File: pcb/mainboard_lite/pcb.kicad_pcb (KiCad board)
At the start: 4 copper layers, 50 x 47 mm, 196 parts, among them J201 Conn_02x05_Odd_Even, J401 FH12-40S-0.5SH, J402 HDMI_A, J403 USB_C_Receptacle_USB2.0, J404 Power Switch, Q401 BSS138, Q402 BSS138, Q403 BSS138, Q404 BSS84, Q406 S8050W, U200 XC6SLX16-FTG256, U401 SY8120, U402 MT3608, U404 SY8120, U405 SY8120, U406 W25Q16JVP, U407 MT9700, U408 MT3608, U409 LGS5148, U410 LGS5148, U411 LM321, U502 MT41K64M16TW, Y201 33MHz

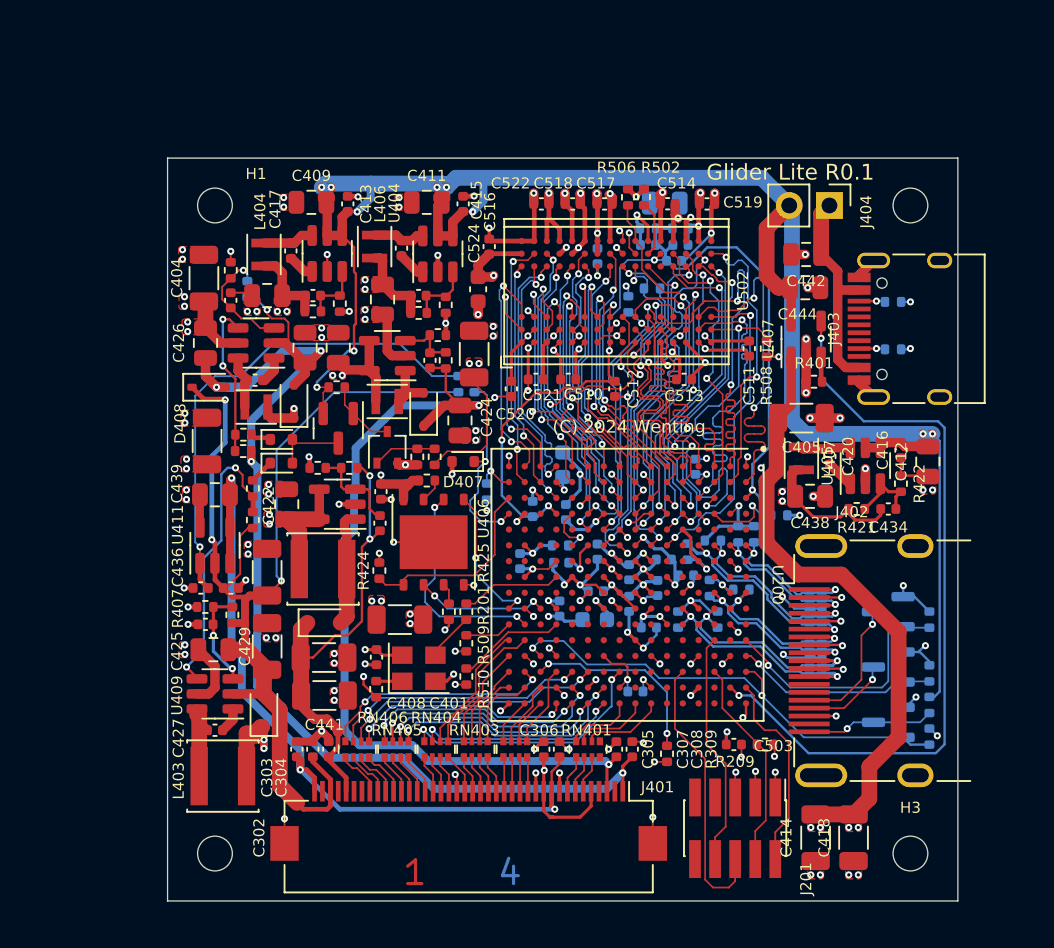
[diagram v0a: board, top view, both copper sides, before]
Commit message: Lite version r0p1
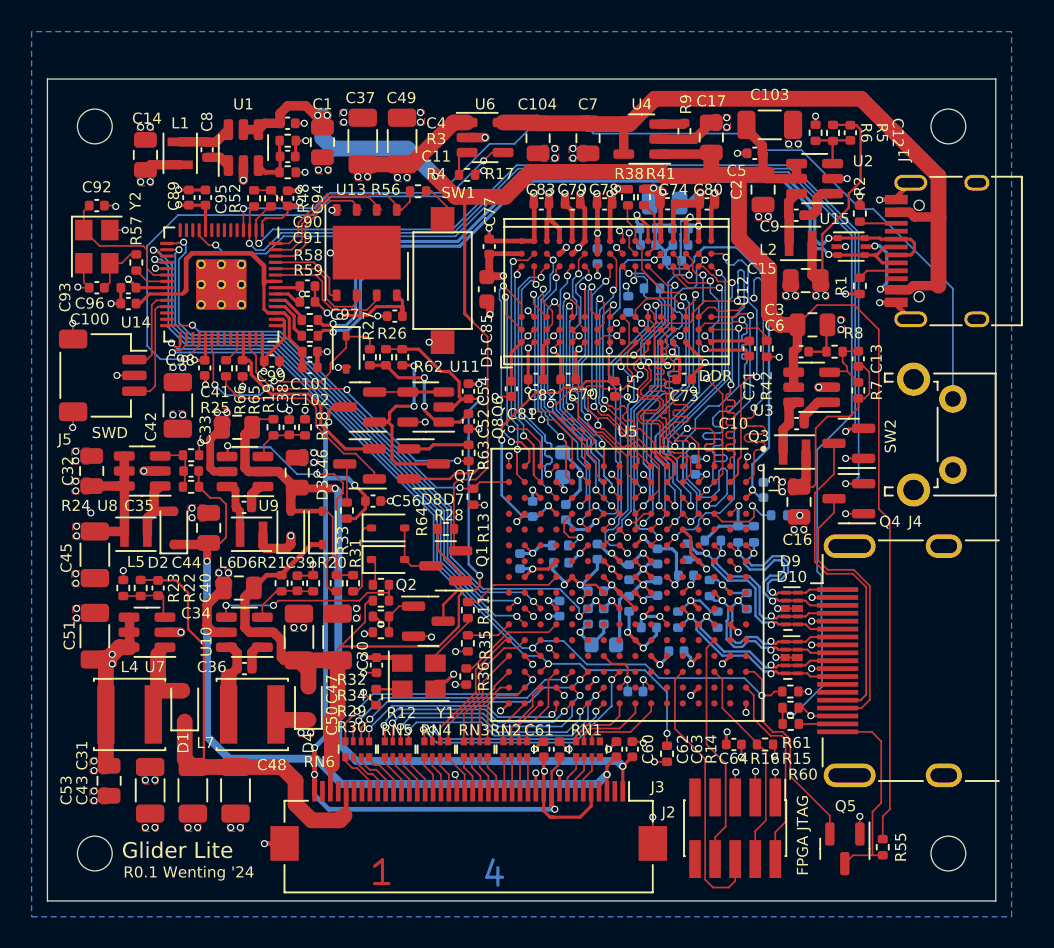
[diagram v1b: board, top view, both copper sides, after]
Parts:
- removed C302, C303, C304, C443: 220nF, Capacitor_SMD:C_0402_1005Metric
- removed C414: 47uF/10V, Capacitor_SMD:C_1206_3216Metric
- removed C442: 10uF/10V, Capacitor_SMD:C_0805_2012Metric
- removed J403: USB_C_Receptacle_USB2.0, Connector_USB:USB_C_Receptacle_HRO_TYPE-C-31-M-12
- removed J404: Power Switch, Connector_PinHeader_2.54mm:PinHeader_1x02_P2.54mm_Vertical
- removed Q401, Q402, Q403: BSS138, Package_TO_SOT_SMD:SOT-23
- removed Q404: BSS84, Package_TO_SOT_SMD:SOT-23
- removed R417, R418: 5.1K/1%, Resistor_SMD:R_0402_1005Metric
- removed R424: 10K/1%, Resistor_SMD:R_0402_1005Metric
- removed R425, R426: 4.7K, Resistor_SMD:R_0402_1005Metric
- removed R428: 1K/1%, Resistor_SMD:R_0402_1005Metric
- removed U402, U408: MT3608, Package_TO_SOT_SMD:TSOT-23-5
- removed U406: W25Q16JVP, Package_SON:WSON-8-1EP_6x5mm_P1.27mm_EP3.4x4.3mm
- added C100: 100nF, Capacitor_SMD:C_0402_1005Metric, F.Cu at (100.1, 62.2)
- added C101: 100nF, Capacitor_SMD:C_0402_1005Metric, F.Cu at (111.6, 65.2)
- added C102: 1uF, Capacitor_SMD:C_0402_1005Metric, F.Cu at (111.6, 66.2)
- added C103: 47uF/10V, Capacitor_SMD:C_1206_3216Metric, F.Cu at (140.7, 50.9)
- added C104: 10uF/10V, Capacitor_SMD:C_0805_2012Metric, F.Cu at (126.0, 51.8)
- added C57: 220nF, Capacitor_SMD:C_0402_1005Metric, B.Cu at (134.8, 84.2)
- added C58: 220nF, Capacitor_SMD:C_0402_1005Metric, B.Cu at (130.2, 82.0)
- added C59: 220nF, Capacitor_SMD:C_0402_1005Metric, B.Cu at (129.2, 82.0)
- added C7: 10uF/10V, Capacitor_SMD:C_0805_2012Metric, F.Cu at (129.2, 51.8)
- added C89: 1uF, Capacitor_SMD:C_0402_1005Metric, F.Cu at (104.0, 55.5)
- added C90: 100nF, Capacitor_SMD:C_0402_1005Metric, F.Cu at (111.5, 61.1)
- added C91: 100nF, Capacitor_SMD:C_0402_1005Metric, F.Cu at (111.5, 62.1)
- added C92: 18pF, Capacitor_SMD:C_0402_1005Metric, F.Cu at (98.1, 56.0)
- added C93: 18pF, Capacitor_SMD:C_0402_1005Metric, F.Cu at (98.1, 61.2)
- added C94: 100nF, Capacitor_SMD:C_0402_1005Metric, F.Cu at (110.2, 55.5)
- added C95: 100nF, Capacitor_SMD:C_0402_1005Metric, F.Cu at (105.0, 55.5)
- added C96: 100nF, Capacitor_SMD:C_0402_1005Metric, F.Cu at (100.1, 61.2)
- added C97: 100nF, Capacitor_SMD:C_0402_1005Metric, F.Cu at (117.0, 63.0)
- added C98: 100nF, Capacitor_SMD:C_0402_1005Metric, F.Cu at (105.0, 66.3)
- added C99: 100nF, Capacitor_SMD:C_0402_1005Metric, F.Cu at (109.2, 65.8)
- added J1: USB_C_Receptacle_USB2.0, Connector_USB:USB_C_Receptacle_HRO_TYPE-C-31-M-12, F.Cu at (152.8, 58.9)
- added J5: SM03B-SRSS-TB, Connector_JST:JST_SH_SM03B-SRSS-TB_1x03-1MP_P1.00mm_Horizontal, F.Cu at (98.5, 66.8)
- added Q1: AO3401A, Package_TO_SOT_SMD:SOT-23, F.Cu at (120.2, 78.8)
- added Q3: AO3400A, Package_TO_SOT_SMD:SOT-23, F.Cu at (145.7, 71.0)
- added Q4: AO3400A, Package_TO_SOT_SMD:SOT-23, F.Cu at (145.7, 74.5)
- added Q5: AO3400A, Package_TO_SOT_SMD:SOT-23, F.Cu at (145.4, 96.7)
- added Q6: AO3400A, Package_TO_SOT_SMD:SOT-23, F.Cu at (114.8, 68.8)
- added Q7: AO3401A, Package_TO_SOT_SMD:SOT-23, F.Cu at (118.8, 72.3)
- added Q8: AO3401A, Package_TO_SOT_SMD:SOT-23, F.Cu at (114.8, 72.3)
- added R1: 5.1K/1%, Resistor_SMD:R_0402_1005Metric, F.Cu at (146.4, 61.1)
- added R15: 1K/1%, Resistor_SMD:R_0402_1005Metric, F.Cu at (142.0, 86.8)
- added R2: 5.1K/1%, Resistor_SMD:R_0402_1005Metric, F.Cu at (146.4, 56.5)
- added R56: 1K, Resistor_SMD:R_0402_1005Metric, F.Cu at (118.5, 55.1)
- added R57: 1K, Resistor_SMD:R_0402_1005Metric, F.Cu at (100.6, 59.6)
- added R58: 27R, Resistor_SMD:R_0402_1005Metric, F.Cu at (111.6, 63.2)
- added R59: 27R, Resistor_SMD:R_0402_1005Metric, F.Cu at (111.6, 64.2)
- added R60: 120K/1%, Resistor_SMD:R_0402_1005Metric, F.Cu at (142.0, 88.8)
- added R61: 240K/1%, Resistor_SMD:R_0402_1005Metric, F.Cu at (142.0, 87.8)
- added R62: 120K/1%, Resistor_SMD:R_0402_1005Metric, F.Cu at (117.5, 65.6)
- added R63: 51R, Resistor_SMD:R_0402_1005Metric, F.Cu at (121.7, 71.7)
- added R64: 20K/1%, Resistor_SMD:R_0402_1005Metric, F.Cu at (114.0, 75.3)
- added R65: 10K/1%, Resistor_SMD:R_0402_1005Metric, F.Cu at (107.3, 66.3)
- added R66: 51R, Resistor_SMD:R_0402_1005Metric, F.Cu at (106.3, 66.3)
- added R9: 10K/1%, Resistor_SMD:R_0402_1005Metric, F.Cu at (135.3, 51.3)
- added SW1: EVQPUJ02K, Button_Switch_SMD:SW_SPST_CK_RS282G05A3, F.Cu at (120.0, 60.8)
- added SW2: SW_Push, Button_Switch_THT:SW_Tactile_SPST_Angled_PTS645Vx58-2LFS, F.Cu at (152.3, 68.2)
- added U13: W25Q32JV, Package_SON:WSON-8-1EP_6x5mm_P1.27mm_EP3.4x4.3mm, F.Cu at (115.2, 59.0)
- added U14: RP2040, footprints:RP2040-QFN-56, F.Cu at (106.0, 61.0)
- added U15: USBLC6-2P6, Package_TO_SOT_SMD:SOT-666, F.Cu at (145.8, 58.6)
- added U4: MT9700, Package_TO_SOT_SMD:SOT-23-5, F.Cu at (132.6, 51.8)
- added U7: MT3608(SOT23-6), Package_TO_SOT_SMD:SOT-23-6, F.Cu at (101.3, 83.0)
- added U8: MT3608(SOT23-6), Package_TO_SOT_SMD:SOT-23-6, F.Cu at (101.0, 72.8)
- added Y2: 12MHz, Oscillator:Oscillator_SMD_Abracon_ASE-4Pin_3.2x2.5mm, F.Cu at (98.1, 58.6)
- C56: renamed from C439; value 10uF/10V -> 1uF; footprint Capacitor_SMD:C_0805_2012Metric -> Capacitor_SMD:C_0402_1005Metric
- D10: renamed from D405; moved to F.Cu
- D5: renamed from D407; value 4148WT -> 4148WS; footprint Diode_SMD:D_SOD-523 -> Diode_SMD:D_SOD-323
- D7: renamed from D410; value 4148WT -> 4148WS; footprint Diode_SMD:D_SOD-523 -> Diode_SMD:D_SOD-323
- D8: renamed from D409; value 4148WT -> 4148WS; footprint Diode_SMD:D_SOD-523 -> Diode_SMD:D_SOD-323
- D9: renamed from D404; moved to F.Cu
- Q2: renamed from Q406; value S8050W -> S8050; footprint Package_TO_SOT_SMD:SOT-323_SC-70 -> Package_TO_SOT_SMD:SOT-23
- R13: renamed from R306; moved to F.Cu
- R17: renamed from R401; value 5.1K/1% -> 10K/1%
- R19: renamed from R409; moved to F.Cu
- R26: renamed from R410; moved to F.Cu
- R27: renamed from R411; moved to F.Cu
- R48: renamed from R412; moved to F.Cu
- R52: renamed from R413; moved to F.Cu
- R55: renamed from R414; moved to F.Cu
- moved R48 51.4 mm to (109.2, 55.5)
- moved R52 50.4 mm to (108.1, 55.5)
- moved C53 44.6 mm to (101.5, 93.0)
- moved C37 32.8 mm to (115.0, 51.9), turned to -90 degrees
- moved C12 29.2 mm to (145.8, 51.4), turned to 90 degrees
- moved R5 28.6 mm to (144.7, 51.4), turned to 90 degrees
- moved C45 27.2 mm to (98.0, 78.1), turned to 90 degrees
- moved L2 27.0 mm to (142.7, 58.4), turned to 0 degrees
- moved C15 26.8 mm to (143.0, 60.8), turned to 0 degrees
- moved R6 25.8 mm to (143.6, 51.4), turned to -90 degrees
- moved R17 25.6 mm to (121.5, 54.1), turned to 180 degrees
- moved C9 25.1 mm to (142.4, 56.6), turned to 0 degrees
- moved U2 24.3 mm to (143.5, 54.3), turned to 180 degrees
- moved U6 24.0 mm to (122.7, 51.7), turned to 0 degrees
- moved C49 22.6 mm to (117.4, 51.9)
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- renumbered C409 to C1, C420 to C10, C421 to C11, C433 to C12, C434 to C13, C435 to C14, C437 to C15, C438 to C16, C444 to C17, C210 to C18, C213 to C19, C411 to C2, C215 to C20, C217 to C21, C219 to C22, C220 to C23, C211 to C24, C214 to C25, C201 to C26, C203 to C27, C204 to C28, C202 to C29, C412 to C3, C209 to C30, C422 to C31, C406 to C32, C426 to C33, C425 to C34, C430 to C35, C427 to C36, C405 to C37, C431 to C38, C428 to C39, C413 to C4, C407 to C40, C423 to C41, C404 to C42, C408 to C43, C424 to C44, C403 to C45, C432 to C46, C429 to C47, C441 to C48, C402 to C49, C415 to C5, C445 to C50, C401 to C51, C436 to C52, C418 to C53, C440 to C54, C416 to C6, C305 to C60, C306 to C61, C307 to C62, C308 to C63, C503 to C64, C501 to C65, C504 to C66, C502 to C67, C529 to C68, C508 to C69, C510 to C70, C511 to C71, C509 to C72, C513 to C73, C514 to C74, C512 to C75, C515 to C76, C516 to C77, C517 to C78, C518 to C79, C417 to C8, C519 to C80, C520 to C81, C521 to C82, C522 to C83, C523 to C84, C524 to C85, C525 to C86, C526 to C87, C527 to C88, C419 to C9, D401 to D1, D402 to D2, D406 to D3, D403 to D4, D408 to D6, J201 to J2, J401 to J3, J402 to J4, L404 to L1, L406 to L2, L407 to L3, L401 to L4, L402 to L5, L405 to L6, L403 to L7, R310 to R10, R201 to R11, R202 to R12, R309 to R14, R209 to R16, R408 to R18, R406 to R20, R407 to R21, R402 to R22, R403 to R23, R404 to R24, R405 to R25, R427 to R28, R429 to R29, R415 to R3, R430 to R30, R431 to R31, R432 to R32, R433 to R33, R434 to R34, R509 to R35, R510 to R36, R505 to R37, R506 to R38, R501 to R39, R416 to R4, R507 to R40, R502 to R41, R508 to R42, R503 to R43, R504 to R44, R423 to R45, R435 to R46, R436 to R47, R437 to R49, R419 to R5, R438 to R50, R439 to R51, R440 to R53, R441 to R54, R420 to R6, R421 to R7, R422 to R8, RN401 to RN1, RN402 to RN2, RN403 to RN3, RN404 to RN4, RN405 to RN5, RN406 to RN6, U401 to U1, U409 to U10, U411 to U11, U502 to U12, U404 to U2, U405 to U3, U200 to U5, U407 to U6, U410 to U9, Y201 to Y1
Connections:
- J4 pad 18: unconnected-(J402-+5V-Pad18) -> Net-(J4-+5V)
- R36 pad 1: GND -> +3V3
- U11 pad 3: VCOM -> Net-(Q6-S)
- U11 pad 4: VCOM -> Net-(Q6-S)
- U5 pad A12: DDC_SCL -> unconnected-(U5A-IO_L62N_VREF_0-PadA12)
- U5 pad A13: DDC_SDA -> unconnected-(U5A-IO_L63N_SCP6_0-PadA13)
- U5 pad B15: EPD_POWEREN -> unconnected-(U5A-IO_L29P_A23_M1A13_1-PadB15)
- U5 pad L10: unconnected-(U200B-IO_L16P_2-PadL10) -> FPGA_CS
- U5 pad P10: FPGA_FMISO -> FPGA_MOSI
- U5 pad R11: FPGA_FCCLK -> FPGA_SCLK
- U5 pad T10: FPGA_FMOSI -> FPGA_MISO
- U5 pad T3: FPGA_FCS -> unconnected-(U5B-IO_L65N_CSO_B_2-PadT3)
- U5 pad T4: EPD_VCOM_PWM -> unconnected-(U5B-IO_L63N_2-PadT4)
- U6 pad 4: EPD_POWEREN -> EPD_PWR_EN
- U6 pad 5: +5V -> VBUS
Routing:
- net HDMI_DET: track 0.00 -> 80.0 mm, vias 0 -> 2
- net KEY: track 0.00 -> 59.5 mm, vias 0 -> 1
- net DDC_SDA: track 12.9 -> 62.3 mm, vias 1 -> 2
- net /mcu/USB_DP: track 0.00 -> 48.3 mm, vias 0 -> 2
- net EPD_POWEREN: track 48.3 -> 0.00 mm, vias 2 -> 0
- net /mcu/USB_DN: track 0.00 -> 47.1 mm, vias 0 -> 2
- net DDC_SCL: track 16.5 -> 58.9 mm, vias 1 -> 2
- net FPGA_CS: track 0.00 -> 42.4 mm, vias 0 -> 2
- net FPGA_MISO: track 0.00 -> 38.1 mm, vias 0 -> 2
- net FPGA_MOSI: track 0.00 -> 38.0 mm, vias 0 -> 2
- net FPGA_SCLK: track 0.00 -> 37.9 mm, vias 0 -> 2
- net VBUS: track 13.4 -> 49.7 mm, vias 0 -> 2
- net EPD_PWR_EN: track 0.00 -> 35.7 mm, vias 0 -> 2
- net FPGA_SUSP: track 12.3 -> 47.6 mm, vias 2 -> 3
- net FPGA_DONE: track 30.9 -> 65.1 mm, vias 2 -> 3
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- added copper zone on B.Cu, net GND
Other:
- board size 50 x 47 mm -> 60 x 52 mm
- board text added: "DDR"
- board text added: "FPGA JTAG"
- board text added: "Glider Lite"
- board text added: "R0.1 Wenting '24"
- board text added: "SWD"
- board text removed: "(C) 2024 Wenting"
- board text removed: "Glider Lite R0.1"
